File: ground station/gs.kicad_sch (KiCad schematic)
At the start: 29 parts, among them J1 USB_C_Receptacle_USB2.0_14P, J2 OLED, J4 H9161TR-ND, U1 ATSAMD21G18A-A, U17 PE4259, U2 SX1262IMLTRT, Y2 32MHz

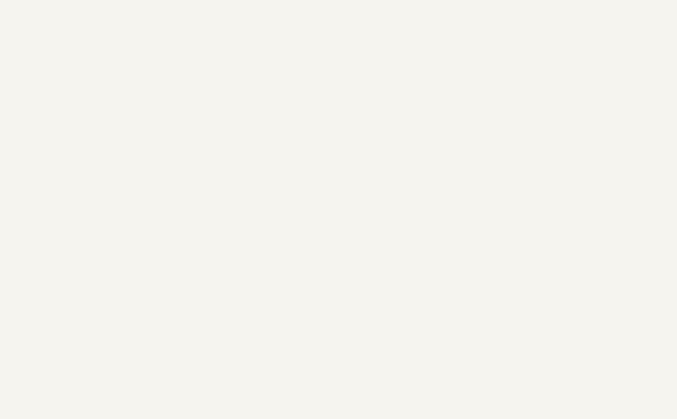
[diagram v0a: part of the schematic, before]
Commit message: thingy for programming
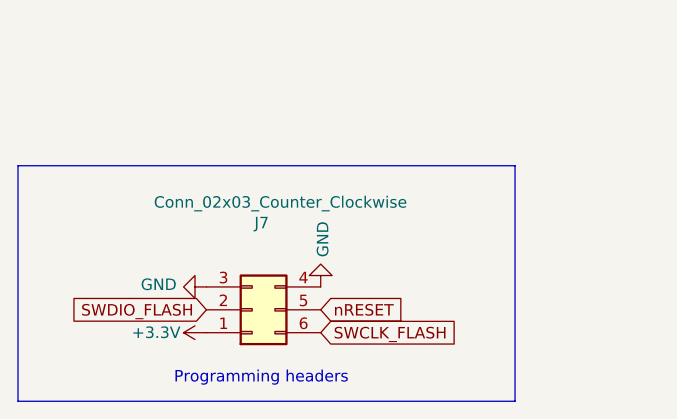
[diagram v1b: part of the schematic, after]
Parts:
- added J7: Conn_02x03_Counter_Clockwise, Connector_PinHeader_2.54mm:PinHeader_2x03_P2.54mm_Vertical, symbol Connector_Generic:Conn_02x03_Counter_Clockwise
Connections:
- net +3.3V: now also J7.1 (Pin_1)
- net GND: now also J7.3 (Pin_3), J7.4 (Pin_4)
- net SWCLK_FLASH: now also J7.6 (Pin_6)
- net SWDIO_FLASH: now also J7.2 (Pin_2)
- net nRESET: now also J7.5 (Pin_5)
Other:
- note added: "Programming headers"
